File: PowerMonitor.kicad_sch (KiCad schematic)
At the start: 59 parts, among them U1 TPS76350, U2 AMC1301 or AMC1302, U3 AMC1301, U4 SN6501DBV, U5 OPA2197IDR, U6 ISL28022

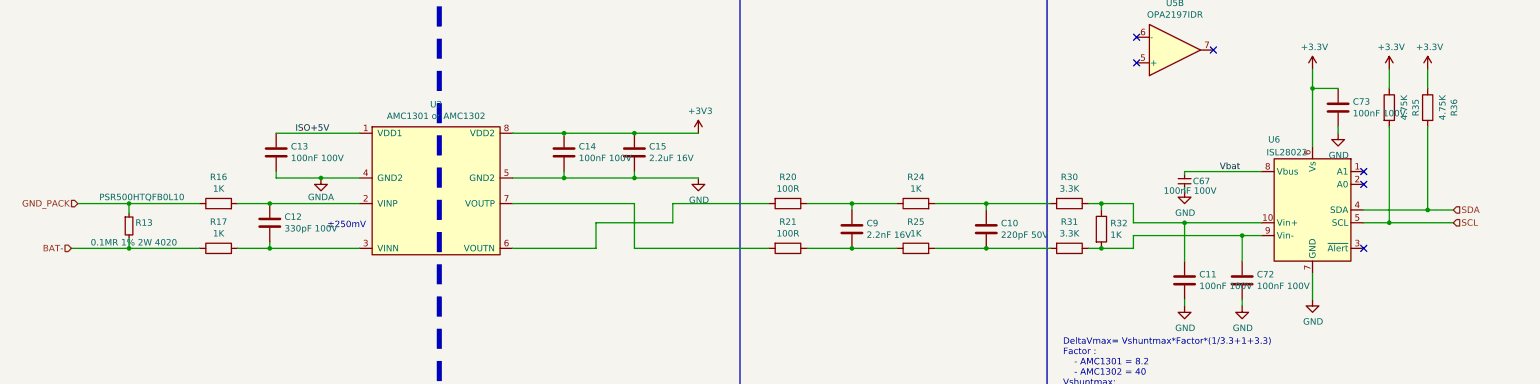
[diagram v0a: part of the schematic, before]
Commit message: Add files via upload
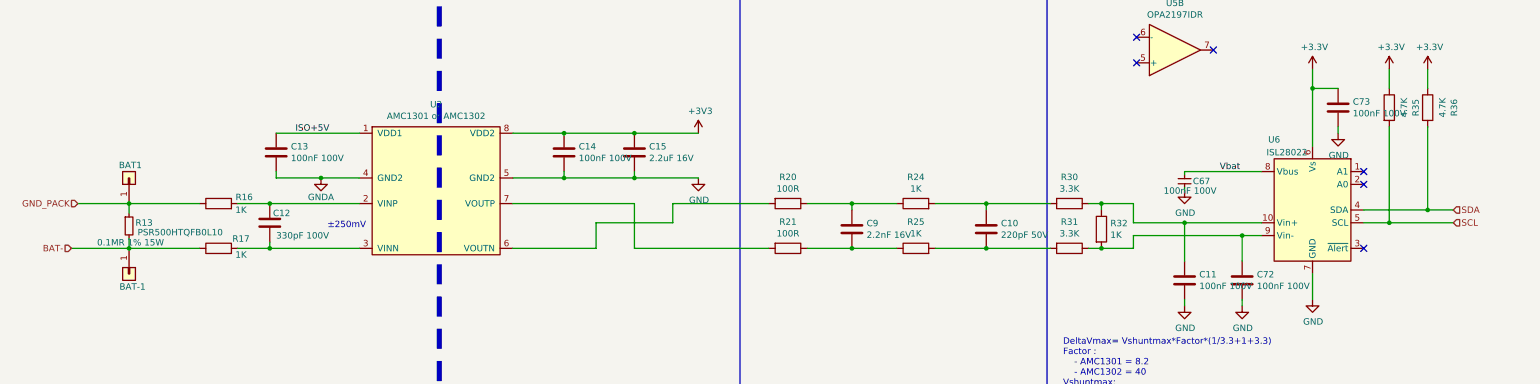
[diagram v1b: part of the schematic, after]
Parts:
- added BAT-1, BAT1: BAT-, Battery:Battery_6mm×10mm_Cell_half_2, symbol Connector_Generic:Conn_01x01
- R10, R19, R28, R29: Link (none) -> https://www.digikey.jp/en/products/detail/yageo/RC0603JR-07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
- R13: value 0.1MR 1% 2W 4020 -> 0.1MR 1% 15W; Link https://www.mouser.jp/ProductDetail/ROHM-Semiconductor/PSR5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 -> https://www.digikey.jp/en/products/detail/rohm-semiconducto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
- R15: Link https://www.digikey.jp/en/products/detail/panasonic-electronic-components/ERJ-PB6B1001V/6213377?s=N4IgTCBcDaIKICUBSAFAQgNjQRgAy%2BwDUQBdAXyA -> https://www.digikey.jp/en/products/detail/panasonic-electronic-components/ERJ-PB6B1001V/6213377?s=N4IgTCBcDaIKICUBSBaACgIQGwYIwAZ9cA1EAXQF8g
- R16, R17, R18, R24, R25, R26, R27, R32: Link (none) -> https://www.digikey.jp/en/products/detail/vishay-dale/CRCW0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; MPN MCR03EZPFX1001 -> CRCW06031K00FKEA
- R20, R21, R22, R23, R30, R31, R33, R34: Link (none) -> https://www.digikey.jp/en/products/detail/yageo/RC0603FR-07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
- R35, R36: value 4.75K -> 4.7K; Link (none) -> https://www.digikey.jp/en/products/detail/yageo/RC0603JR-07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
- TR1: Link (none) -> https://www.digikey.jp/en/products/detail/w%C3%BCrth-elektr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
- U1, U2, U4, U5: Link (none) -> https://www.digikey.jp/en/products/detail/texas-instruments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
- U5: footprint Housings_SOIC:SOIC-8_3.9x4.9mm_Pitch1.27mm -> PCM_4ms_Package_SOIC:SOIC-8_3.9x4.9mm_Pitch1.27mm; Link (none) -> https://www.digikey.jp/en/products/detail/texas-instruments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
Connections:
- net BAT-: now also BAT-1.1 (Pin_1)
- net GND_PACK: now also BAT1.1 (Pin_1)
